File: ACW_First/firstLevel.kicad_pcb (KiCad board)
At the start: 2 copper layers, 103 x 65 mm, 75 parts, among them J1 Screw_Terminal_01x02, J10 Conn_01x04_Pin, J6 Screw_Terminal_01x02, J7 Screw_Terminal_01x04, J8 Conn_01x02_Pin, J9 Conn_01x03_Socket, K1 SRD-05VDC-SL-C, Q1 S8050, U4 PC817, U5 HT7133-1_C15060, U6 V9881D, U7 CT817C, U8 CT817C

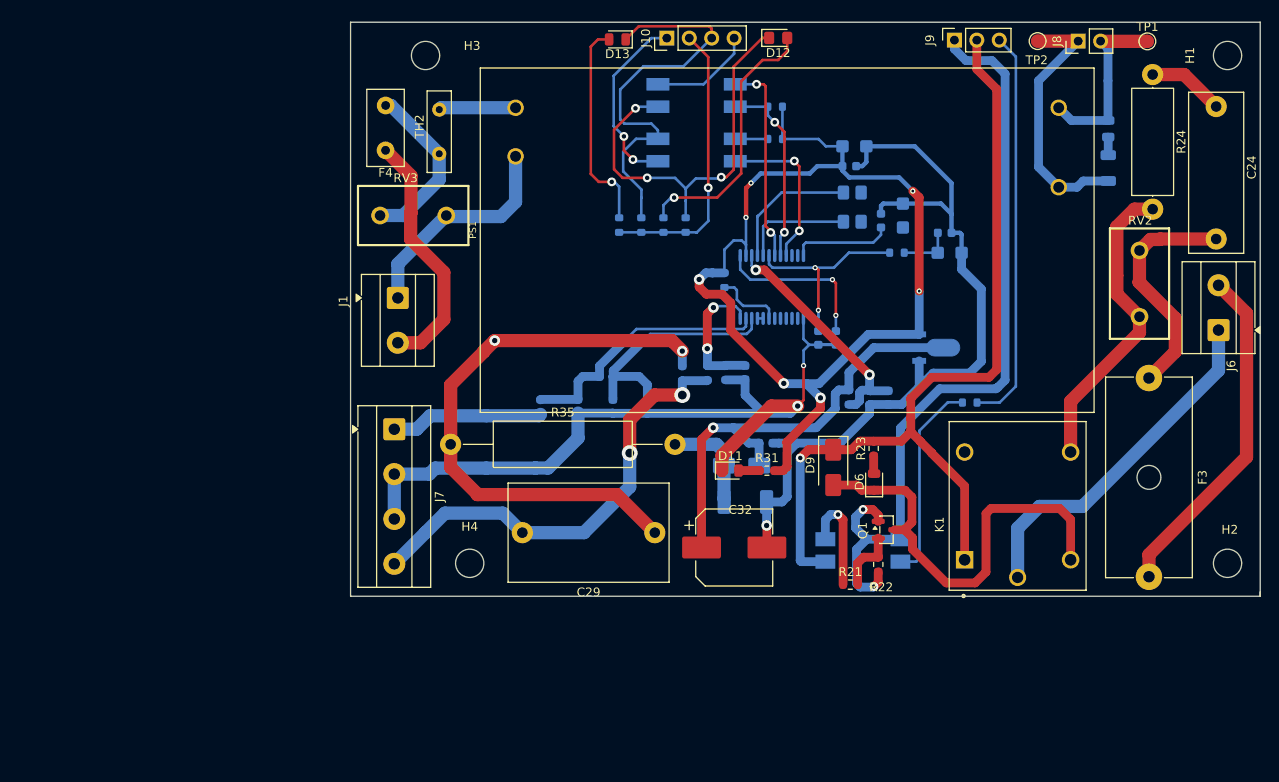
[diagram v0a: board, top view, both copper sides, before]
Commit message: revisi
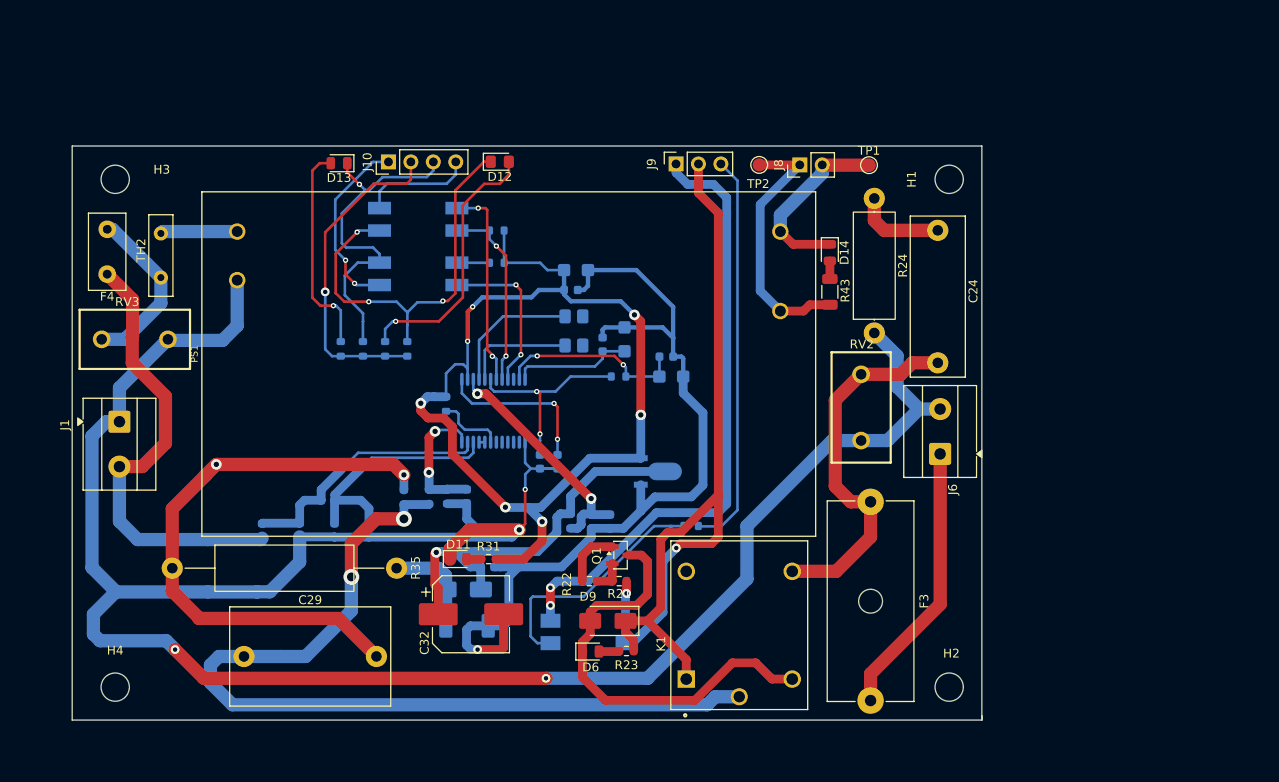
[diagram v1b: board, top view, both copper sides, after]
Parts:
- removed J7: Screw_Terminal_01x04, TerminalBlock_MetzConnect:TerminalBlock_MetzConnect_Type101_RT01604HBWC_1x04_P5.08mm_Horizontal
- removed U4: PC817, Custom_Library:SOP254P975X460-4N
- added U1: PC817, Custom_Library:SOP254P975X460-4N, B.Cu at (415.2, 238.3)
- D14, R43: moved to F.Cu
- moved H4 42.5 mm to (361.6, 244.5)
- moved H3 37.8 mm to (361.6, 187.0)
- moved D6 37.4 mm to (415.5, 240.5), turned to 0 degrees
- moved R23 36.2 mm to (419.5, 240.4), turned to 0 degrees
- moved R20 34.5 mm to (426.8, 226.3)
- moved C27 34.5 mm to (385.7, 223.4)
- moved C28 34.5 mm to (401.4, 222.9)
- moved C29 34.5 mm to (391.2, 241.1)
- moved C30 34.5 mm to (411.7, 219.0)
- moved C31 34.5 mm to (403.8, 230.9)
- moved C34 34.5 mm to (413.8, 197.3)
- moved C36 34.5 mm to (424.6, 209.4)
- moved C37 34.5 mm to (413.2, 199.6)
- moved C38 34.5 mm to (416.8, 205.7)
- moved C40 34.5 mm to (409.7, 219.0)
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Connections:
- net /LIVE to 24V/24VDC renamed /24VDC
- C25 pad 1: /PZEM/CT2 -> /Neutral
- C26 pad 1: /PZEM/CT2 -> /Neutral
- C28 pad 2: /PZEM/CT2 -> /Neutral
- C29 pad 2: /PZEM/L -> /Live_OutPZEM
- C30 pad 2: /PZEM/CT2 -> /Neutral
- C40 pad 2: /PZEM/CT2 -> /Neutral
- D11 pad 1: /PZEM/CT2 -> /Neutral
- J6 pad 1: /Relay/COM -> /Relay/NO
- J6 pad 2: /Relay/NO -> /Neutral
- K1 pad COM: /Relay/COM -> /Live_OutPZEM
- K1 pad NO: Net-(K1-PadNO) -> Net-(C24-Pad1)
- R24 pad 1: Net-(K1-PadNO) -> /Neutral
- R25 pad 1: /PZEM/CT2 -> /Neutral
- R25 pad 2: /PZEM/CT1 -> /Live
- R26 pad 1: /PZEM/CT1 -> /Live
- R27 pad 1: /PZEM/CT2 -> /Neutral
- R28 pad 2: /PZEM/L -> /Live_OutPZEM
- R29 pad 1: /PZEM/CT2 -> /Neutral
- R30 pad 1: /PZEM/L -> /Live_OutPZEM
- RV2 pad 2: Net-(K1-PadNO) -> /Neutral
- U6 pad 13: /PZEM/CT2 -> /Neutral
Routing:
- net /Neutral: track 25.3 -> 261.3 mm, vias 0 -> 4
- net /Live_OutPZEM: track 0.00 -> 101.2 mm, vias 0 -> 2
- net /PZEM/CT2: track 90.8 -> 0.00 mm, vias 2 -> 0
- net /PZEM/L: track 51.4 -> 0.00 mm, vias 2 -> 0
- net /Relay/COM: track 40.3 -> 0.00 mm
- net Net-(K1-PadNO): track 34.7 -> 0.00 mm
- net /Live: track 28.2 -> 51.6 mm
- net /PZEM/CT1: track 17.3 -> 0.00 mm
- net Net-(C24-Pad1): track 26.6 -> 42.3 mm
- net Net-(U6-P1.3/RXD5/INT0/CFx/SP/PLLDIV/WAKEUP2): track 6.06 -> 21.6 mm, vias 0 -> 2
- net GND: track 131.5 -> 119.0 mm
- net /Relay/NO: track 38.9 -> 31.2 mm
- net AGND: track 91.4 -> 98.9 mm
- net Net-(R21-Pad1): track 12.0 -> 4.53 mm
- net /PZEM/U7/4OUT: track 46.3 -> 39.2 mm, vias 0 -> 1
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
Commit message: okok
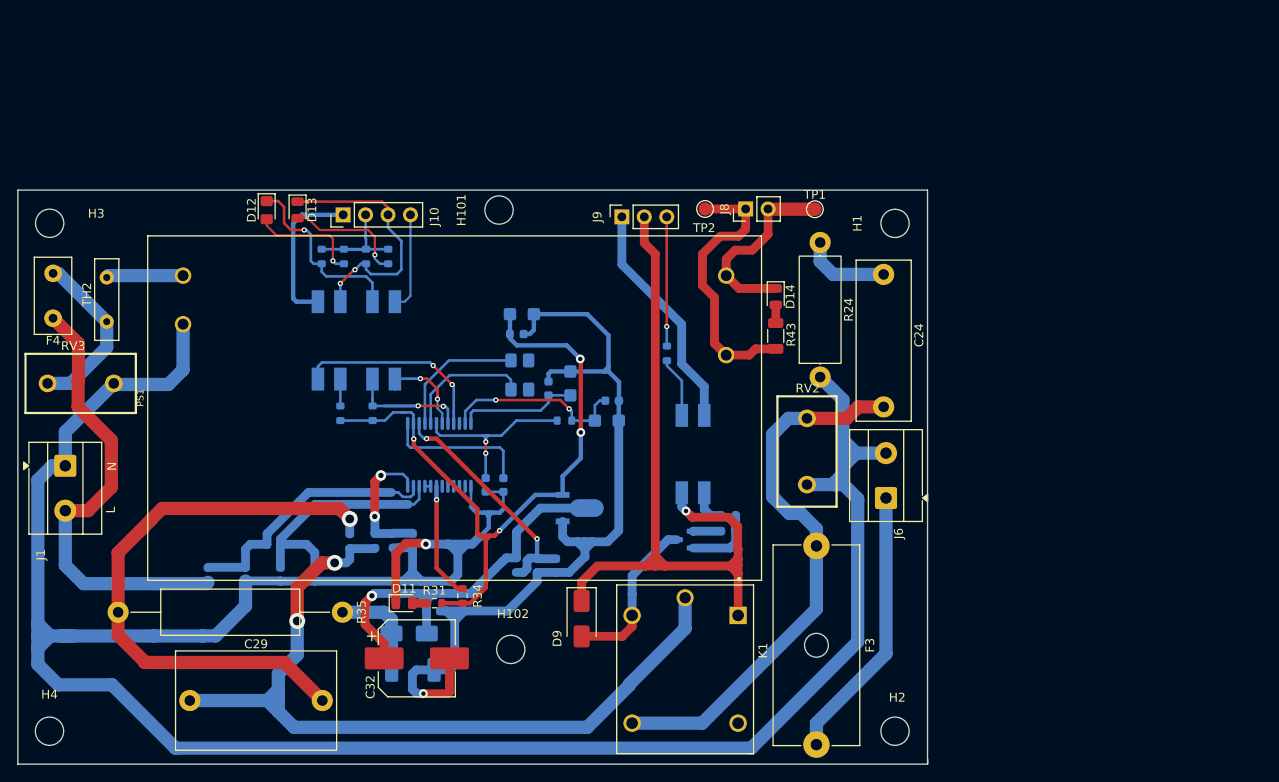
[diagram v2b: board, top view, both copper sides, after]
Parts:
- removed D6: LED_Red, LED_SMD:LED_0805_2012Metric
- removed R23: 1KΩ, Resistor_SMD:R_0603_1608Metric
- added H101: MountingHole, MountingHole:MountingHole_3.2mm_M3, F.Cu at (405.1, 190.5)
- added H102: MountingHole, MountingHole:MountingHole_3.2mm_M3, F.Cu at (406.4, 240.2)
- Q1, R21, R22: moved to B.Cu
- R34: moved to F.Cu
- U1: footprint Custom_Library:SOP254P975X460-4N -> Custom_Footprints:SOP-4_L6.4-W4.6-P2.54-LS10.2-TL
- moved D12 27.0 mm to (378.8, 190.5), turned to -90 degrees
- moved R37 25.0 mm to (390.8, 213.5), turned to 90 degrees
- moved R38 24.6 mm to (387.1, 213.5), turned to -90 degrees
- moved U1 23.4 mm to (427.1, 218.1), turned to -90 degrees
- moved R34 21.8 mm to (400.9, 234.2), turned to -90 degrees
- moved R20 19.7 mm to (424.1, 206.7), turned to -90 degrees
- moved R22 16.7 mm to (431.1, 226.9)
- moved R21 14.4 mm to (431.1, 225.1), turned to 0 degrees
- moved R39 14.3 mm to (385.0, 195.8), turned to -90 degrees
- moved U8 14.3 mm to (392.0, 205.3), turned to -90 degrees
- moved U7 12.6 mm to (385.8, 205.3), turned to 90 degrees
- moved R42 11.8 mm to (392.5, 195.8), turned to -90 degrees
- moved R40 11.5 mm to (387.5, 195.8), turned to -90 degrees
- moved R41 10.5 mm to (390.0, 195.8), turned to -90 degrees
- moved U5 9.78 mm to (413.6, 224.2)
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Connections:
- R38 pad 1: Net-(U5-Vout) -> Net-(U7-ANODE)
- R38 pad 2: Net-(U7-ANODE) -> Net-(U5-Vout)
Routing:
- net GND: track 119.0 -> 69.2 mm, vias 4 -> 0
- net /Neutral: track 261.3 -> 301.4 mm, vias 4 -> 1
- net Net-(U5-Vout): track 112.4 -> 78.2 mm, vias 7 -> 4
- net /Relay/IO_PIN: track 45.1 -> 14.6 mm, vias 0 -> 1
- net Net-(D9-A): track 48.6 -> 18.7 mm
- net /PZEM/U8/1OUT: track 46.2 -> 21.3 mm, vias 3 -> 1
- net /PZEM/5VDC: track 37.0 -> 14.0 mm, vias 1 -> 0
- net Net-(R20-Pad2): track 27.8 -> 7.03 mm
- net Net-(C24-Pad1): track 42.3 -> 62.7 mm
- net Net-(D12-A): track 30.3 -> 12.7 mm
- net Net-(U6-P0.0/TDO): track 23.2 -> 10.6 mm
- net Net-(D13-A): track 24.2 -> 13.9 mm
- net /PZEM/U7/4OUT: track 39.2 -> 29.1 mm, vias 1 -> 2
- net /Relay/5V: track 95.2 -> 85.4 mm
- net /Live_OutPZEM: track 101.2 -> 95.0 mm
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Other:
- board text added: "L"
- board text added: "N"
